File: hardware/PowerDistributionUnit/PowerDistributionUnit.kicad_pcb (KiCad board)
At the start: 2 copper layers, 99.1 x 60.2 mm, 101 parts, among them J1 973582101, J2 973582100, J3 973582101, J4 973582100, Q1 SQJ141ELP, Q2 CSD18511Q5A, SW1 SW_Push, U1 TPS25983, U2 AD5258, U3 NUCLEO_L432KC

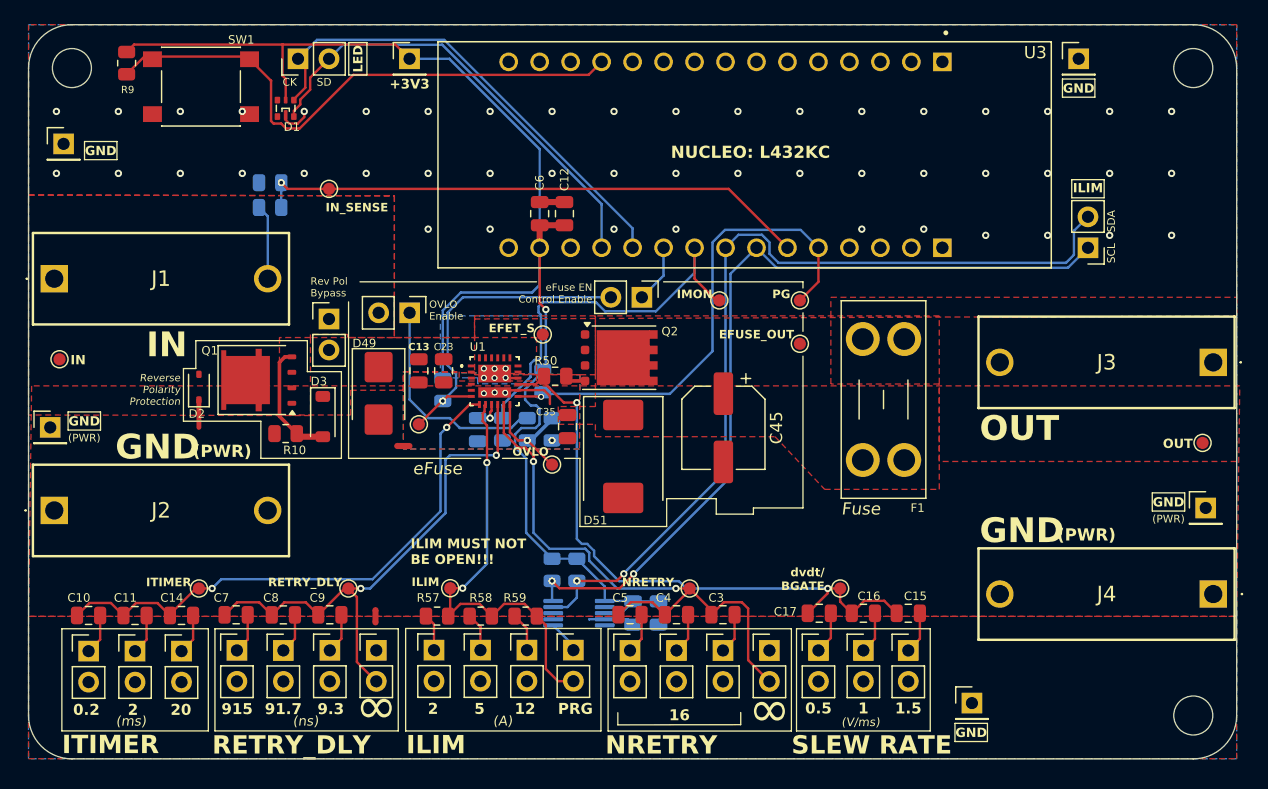
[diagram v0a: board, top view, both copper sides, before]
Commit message: changed led, maybe some other stuff
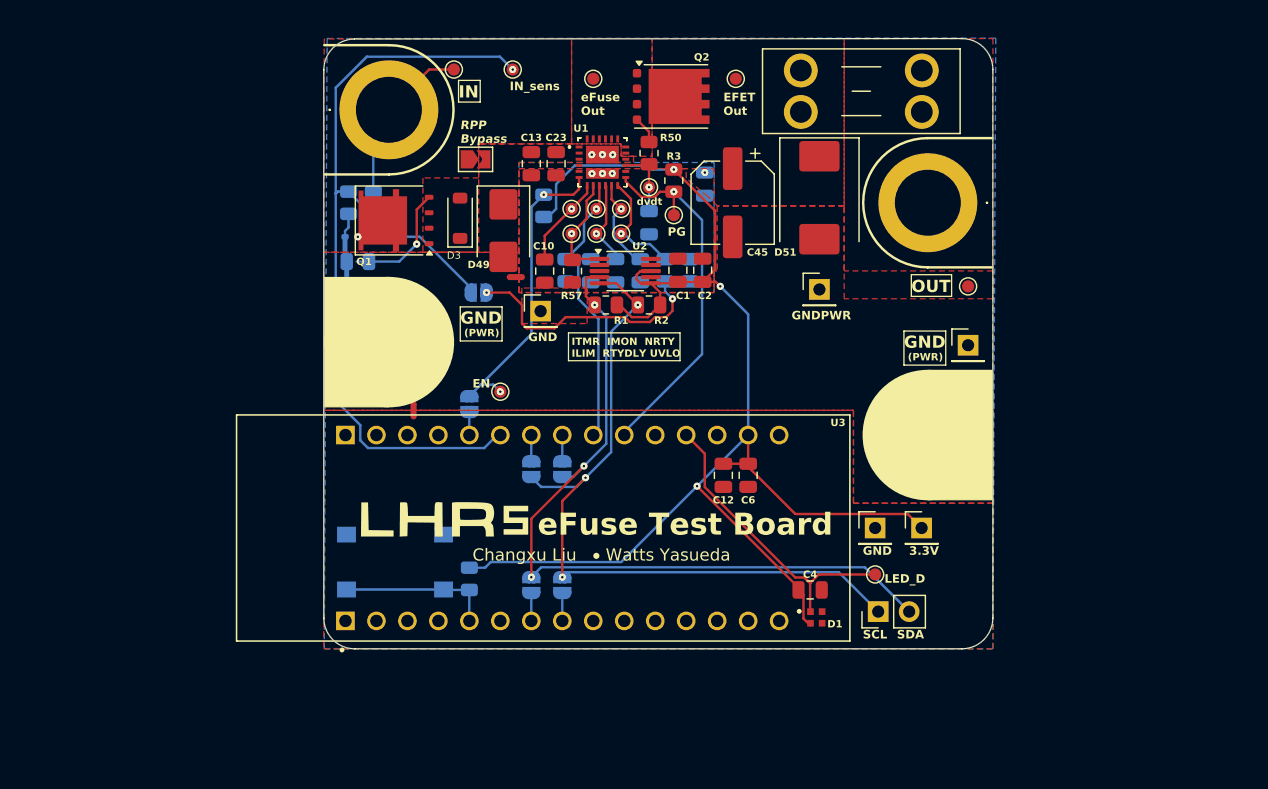
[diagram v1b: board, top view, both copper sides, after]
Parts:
- removed C11, C16: 4.7n, Capacitor_SMD:C_0805_2012Metric
- removed C14: 47n, Capacitor_SMD:C_0805_2012Metric
- removed C17: 10n, Capacitor_SMD:C_0805_2012Metric
- removed C5, C8: 2.2n, Capacitor_SMD:C_0805_2012Metric
- removed C9: 220p, Capacitor_SMD:C_0805_2012Metric
- removed H1, H2, H3: MountingHole, MountingHole:MountingHole_3.2mm_M3
- removed JP11: 200 us, Connector_PinHeader_2.54mm:PinHeader_1x02_P2.54mm_Vertical
- removed JP12: 2 ms, Connector_PinHeader_2.54mm:PinHeader_1x02_P2.54mm_Vertical
- removed JP13: 20 ms, Connector_PinHeader_2.54mm:PinHeader_1x02_P2.54mm_Vertical
- removed JP14: 1.5 V/ms, Connector_PinHeader_2.54mm:PinHeader_1x02_P2.54mm_Vertical
- removed JP15: 1 V/ms, Connector_PinHeader_2.54mm:PinHeader_1x02_P2.54mm_Vertical
- removed JP16: 0.5 V/ms, Connector_PinHeader_2.54mm:PinHeader_1x02_P2.54mm_Vertical
- removed JP17: Latching, Connector_PinHeader_2.54mm:PinHeader_1x02_P2.54mm_Vertical
- removed JP18: Inf, Connector_PinHeader_2.54mm:PinHeader_1x02_P2.54mm_Vertical
- removed JP6: 16 (9.3 ms), Connector_PinHeader_2.54mm:PinHeader_1x02_P2.54mm_Vertical
- removed JP7: 915 ms, Connector_PinHeader_2.54mm:PinHeader_1x02_P2.54mm_Vertical
- removed JP79: ~2A, Connector_PinHeader_2.54mm:PinHeader_1x02_P2.54mm_Vertical
- removed JP8: 91.7 ms, Connector_PinHeader_2.54mm:PinHeader_1x02_P2.54mm_Vertical
- removed JP80: ~5A, Connector_PinHeader_2.54mm:PinHeader_1x02_P2.54mm_Vertical
- removed JP81: ~12A, Connector_PinHeader_2.54mm:PinHeader_1x02_P2.54mm_Vertical
- removed JP9: 9.3 ms, Connector_PinHeader_2.54mm:PinHeader_1x02_P2.54mm_Vertical
- removed R58: 294, Resistor_SMD:R_0805_2012Metric
- removed R59: 121, Resistor_SMD:R_0805_2012Metric
- removed TP14: GND, Connector_PinHeader_2.54mm:PinHeader_1x01_P2.54mm_Vertical
- added JP3: JP, Jumper:SolderJumper-2_P1.3mm_Open_RoundedPad1.0x1.5mm, B.Cu at (132.1, 107.2)
- C1, C2, G***, R1, R2, R3, U2: moved to F.Cu
- C15, C3, C35, C7, D2, R10, R9, SW1: moved to B.Cu
- C4: value 22n -> 0.1u
- D1: value 587-1016-247F -> SK6085; footprint PowerDistributionUnitLib:587-1016-247F -> PowerDistributionUnitLib:SK6085
- J1, J3: footprint PowerDistributionUnitLib:973582101 -> PowerDistributionUnitLib:5754
- J2, J4: footprint PowerDistributionUnitLib:973582100 -> PowerDistributionUnitLib:5754
- JP1, JP19, JP77: footprint Connector_PinHeader_2.54mm:PinHeader_1x02_P2.54mm_Vertical -> Jumper:SolderJumper-2_P1.3mm_Open_RoundedPad1.0x1.5mm; moved to B.Cu
- JP2: footprint Connector_PinHeader_2.54mm:PinHeader_1x02_P2.54mm_Vertical -> Jumper:SolderJumper-2_P1.3mm_Open_TrianglePad1.0x1.5mm
- JP4: value 16 (915 ms) -> JP; footprint Connector_PinHeader_2.54mm:PinHeader_1x02_P2.54mm_Vertical -> Jumper:SolderJumper-2_P1.3mm_Open_RoundedPad1.0x1.5mm; moved to B.Cu
- JP5: value 16 (91.7 ms) -> JP; footprint Connector_PinHeader_2.54mm:PinHeader_1x02_P2.54mm_Vertical -> Jumper:SolderJumper-2_P1.3mm_Open_RoundedPad1.0x1.5mm; moved to B.Cu
- TP10: value Conn_01x02 -> IN_SENSE; footprint Connector_PinHeader_2.54mm:PinHeader_1x02_P2.54mm_Vertical -> TestPoint:TestPoint_Pad_D1.0mm
- moved TP8 64.1 mm to (155.7, 92.5)
- moved TP10 63.5 mm to (160.3, 115.8), turned to 0 degrees
- moved G*** 61.3 mm to (125.0, 111.3), turned to 0 degrees
- moved D1 60.3 mm to (155.4, 119.3)
- moved TP4 56.9 mm to (164.1, 112.0)
- moved R9 50.8 mm to (127.0, 116.2)
- moved TP6 47.8 mm to (132.8, 94.2)
- moved C10 46.9 mm to (133.2, 90.9), turned to 90 degrees
- moved TP3 43.6 mm to (135.4, 85.9)
- moved SW1 42.1 mm to (120.9, 114.8)
- moved C7 42.0 mm to (139.0, 90.9), turned to 90 degrees
- moved TP5 41.9 mm to (160.3, 112.0)
- moved TP76 40.1 mm to (125.7, 74.4)
- moved C15 38.4 mm to (141.7, 87.0), turned to 90 degrees
- moved TP1 36.4 mm to (141.7, 84.1)
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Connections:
- C10 pad 1: Net-(JP11-A) -> GND
- C15 pad 1: Net-(JP14-A) -> GND
- C3 pad 1: Net-(JP4-A) -> GND
- C4 pad 1: Net-(JP5-A) -> +3V3
- C4 pad 2: /NRETRY -> GND
- C7 pad 1: Net-(JP7-A) -> GND
- D1 pad 1: GND -> /LED_D
- D1 pad 2: unconnected-(D1-SDO-Pad2) -> +3V3
- D1 pad 4: +3V3 -> GND
- JP1 pad 2: /ILIM -> /ILIM_SDA
- JP4 pad 2: GND -> /ILIM_SCL
- JP5 pad 2: GND -> /ILIM_SDA
- R57 pad 1: Net-(JP79-A) -> GND
- R8 pad 2: GND -> GNDPWR
- TP10 pad 1: /LED_CK -> /LED_D
- U2 pad 1: Net-(JP1-A) -> /ILIM
- U3 pad CN3_12: /IND_BTN -> unconnected-(U3-PA8-PadCN3_12)
- U3 pad CN3_5: unconnected-(U3-PA12-PadCN3_5) -> /IND_BTN
- U3 pad CN3_7: unconnected-(U3-PB7-PadCN3_7) -> Net-(JP5-A)
- U3 pad CN3_8: unconnected-(U3-PB6-PadCN3_8) -> Net-(JP4-A)
- U3 pad CN4_10: Net-(JP19-A) -> /PG
- U3 pad CN4_11: /LED_CK -> unconnected-(U3-PA1-PadCN4_11)
- U3 pad CN4_12: /LED_SD -> /LED_D
- U3 pad CN4_5: /PG -> Net-(JP19-A)
- U3 pad CN4_7: /ILIM_SCL -> Net-(JP3-A)
- U3 pad CN4_8: /ILIM_SDA -> Net-(JP1-A)
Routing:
- net /dVdt/BGATE: track 50.7 -> 5.78 mm, vias 2 -> 1
- net /NRETRY: track 47.8 -> 7.70 mm, vias 2 -> 1
- net /LED_CK: track 40.1 -> 0.00 mm
- net /ITIMER: track 45.6 -> 7.50 mm, vias 2 -> 1
- net /RETRY_DLY: track 44.8 -> 7.03 mm, vias 2 -> 1
- net /LED_SD: track 37.7 -> 0.00 mm
- net /IND_BTN: track 46.7 -> 12.7 mm
- net /ILIM: track 35.9 -> 9.11 mm, vias 2 -> 1
- net /LED_D: track 0.00 -> 25.3 mm
- net /IN: track 6.32 -> 28.6 mm, vias 0 -> 1
- net /IN_SENSE: track 45.7 -> 61.6 mm
- net GND: track 14.0 -> 0.00 mm, vias 52 -> 3
- net /IMON: track 35.9 -> 24.6 mm
- net /PG: track 41.4 -> 30.5 mm
- net GNDPWR: track 2.25 -> 12.1 mm
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- removed copper zone on B.Cu, net /EFUSE_IN
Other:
- board size 99.1 x 60.2 mm -> 54.9 x 50 mm
- board text added: "3.3V"
- board text added: "EFET Out"
- board text added: "EN"
- board text added: "EN PIN"
- board text added: "GNDPWR"
- board text added: "IN_sens"
- board text added: "ITMR IMON NRTY ILIM RTYDLY UVLO"
- board text added: "LED_D"
- board text added: "OVLO EN"
- board text added: "RPP Bypass"
- board text added: "Watts Yasueda"
- board text added: "dvdt"
- board text added: "eFuse Out"
- board text removed: "(A)"
- board text removed: "(V/ms)"
- board text removed: "(ms)"
- board text removed: "(ns)"
- board text removed: "+3V3"
- board text removed: "0.2"
- board text removed: "0.5"
- board text removed: "1"
- board text removed: "1.5"
- board text removed: "12"
- board text removed: "16"
- board text removed: "2"
- board text removed: "20"
- board text removed: "5"
- board text removed: "9.3"
- board text removed: "91.7"
- board text removed: "915"
- board text removed: "C9"
- board text removed: "CK"
- board text removed: "EFET_S"
- board text removed: "EFUSE_OUT"
- board text removed: "Fuse"
- board text removed: "ILIM"
- board text removed: "ILIM MUST NOT BE OPEN!!!"
- board text removed: "IMON"
- board text removed: "IN_SENSE"
- board text removed: "ITIMER"
- board text removed: "LED"
- board text removed: "NRETRY"
- board text removed: "NUCLEO: L432KC"
- board text removed: "OVLO"
- board text removed: "OVLO Enable"
- board text removed: "PRG"
- board text removed: "RETRY_DLY"
- board text removed: "Rev Pol Bypass"
- board text removed: "Reverse Polarity Protection"
- board text removed: "SD"
- board text removed: "SLEW RATE"
- board text removed: "Wataru Yasueda"
- board text removed: "dvdt/ BGATE"
- board text removed: "eFuse"
- board text removed: "eFuse EN Control Enable"
- board text removed: "∞"
